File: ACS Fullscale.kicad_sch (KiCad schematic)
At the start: 18 parts, among them J1 Pulse-20, J2 Conn_01x02, U1 SN65HVD230, U11 R-78E5.0-1.0, U2 MS5611-01BA, U4 Teensy4.1, U5 TPS62202DBV, U6 BHI360, U7 TXS0108EPW

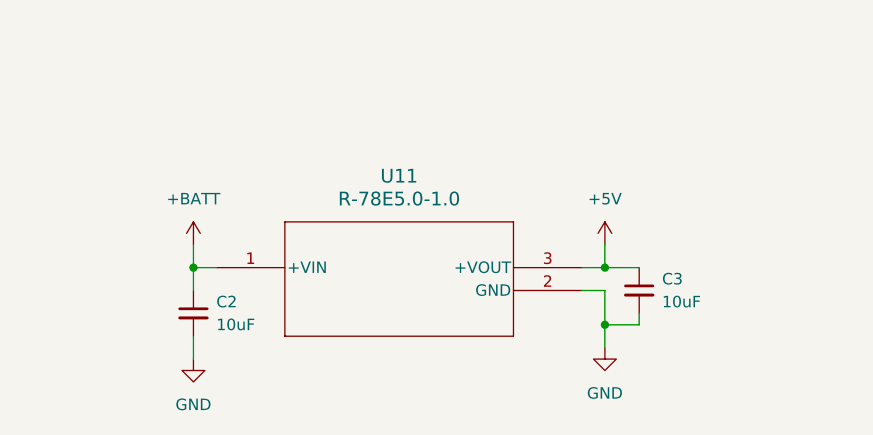
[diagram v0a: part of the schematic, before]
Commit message: fix lib
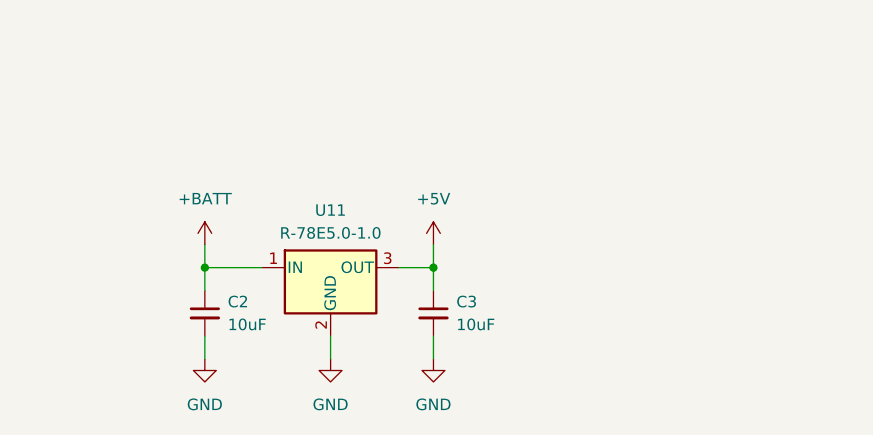
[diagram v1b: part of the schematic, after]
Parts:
- removed J1: Pulse-20, Sensor_Motion:Pulse-20, symbol Sensor_Motion:Pulse-20
- removed U11: R-78E5.0-1.0, R-78E5.0-1.0:R-78C&slash_E-1.0_SIP3_11.6X8.5X10.4_RCP, symbol R-78E5.0-1.0:R-78E5.0-1.0
- removed U4: Teensy4.1, teensy:Teensy41, symbol teensy:Teensy4.1
- removed U6: BHI360, Sensor_Motion:BHI360 Shuttle Board, symbol Sensor_Motion:BHI360_Shuttle_Board
- added J1: Pulse-20, ACS_Footprint_Library:Pulse-20, symbol ACS_symbol_Library:Pulse-20
- added U11: R-78E5.0-1.0, Converter_DCDC:Converter_DCDC_RECOM_R-78E-0.5_THT, symbol Regulator_Switching:R-78E5.0-1.0
- added U4: Teensy4.1, ACS_Footprint_Library:Teensy41, symbol ACS_symbol_Library:Teensy4.1
- added U6: BHI360, ACS_Footprint_Library:BHI360 Shuttle Board, symbol ACS_symbol_Library:BHI360_Shuttle_Board
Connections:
- net +1V8: now also U6.JP1_1 (VDD), U6.JP1_2 (VDDIO)
- net +3V3: now also U4.15 (3V3), U4.46 (3V3)
- net +5V: now also J1.6 (VIN), U11.3 (OUT), U4.48 (VIN)
- net +BATT: now also U11.1 (IN)
- net BT3: now also U4.26 (34_RX8)
- net CANH: now also J1.5 (CAN_H)
- net CANL: now also J1.10 (CAN_L)
- net CANRX: now also U4.45 (23_A9_CRX1_MCLK1)
- net CANTX: now also U4.44 (22_A8_CTX1)
- net CS0: now also U4.12 (10_CS_MQSR)
- net CS1: now also U4.20 (28_RX7)
- net CS2: now also U4.29 (37_CS)
- net CS3: now also U4.28 (36_CS)
- net CS_1V8: now also U6.JP2_1 (CS)
- net GND: now also J1.1 (GND), U11.2 (GND), U4.1 (GND), U4.34 (GND), U4.47 (GND), U6.JP1_3 (GND)
- net INT0: now also U4.11 (9_OUT1C)
- net INT2: now also U4.32 (40_A16)
- net INT3: now also U4.25 (33_MCLK2)
- net INT_1V8: now also U6.JP1_6 (GPIO2/INT1)
- net MISO0: now also U4.14 (12_MISO_MQSL)
- net MISO1: now also U4.3 (1_TX1_CTX2_MISO1)
- net MISO_1V8: now also U6.JP2_3 (SDO)
- net MOSI0: now also U4.13 (11_MOSI_CTX1)
- net MOSI1: now also U4.18 (26_A12_MOSI1)
- net MOSI_1V8: now also U6.JP2_4 (SDI/SDA)
- net RST2: now also U4.33 (41_A17)
- net RST3: now also U4.27 (35_TX8)
- net RST_1V8: now also U6.JP1_5 (GPIO1)
- net SCK0: now also U4.35 (13_SCK_LED)
- net SCK1: now also U4.19 (27_A13_SCK1)
- net SCK_1V8: now also U6.JP2_2 (SCK/SCL)
- net WAKE3: now also U4.24 (32_OUT1B)
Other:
- moved on the sheet: C2, C3
